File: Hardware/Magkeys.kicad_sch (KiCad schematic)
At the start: 206 parts, among them J1 Conn_01x04_Pin, SW1 SW_Push, SW10 SW_Push, SW100 SW_Push, SW101 SW_Push, SW102 RotaryEncoder, SW11 SW_Push, SW12 SW_Push, SW13 SW_Push, SW14 SW_Push, SW15 SW_Push, SW16 SW_Push, SW17 SW_Push, SW18 SW_Push, SW19 SW_Push, SW2 SW_Push, SW20 SW_Push, SW21 SW_Push, SW22 SW_Push, SW23 SW_Push, SW24 SW_Push, SW25 SW_Push, SW26 SW_Push, SW27 SW_Push, SW28 SW_Push, SW29 SW_Push, SW3 SW_Push, SW30 SW_Push, SW31 SW_Push, SW32 SW_Push, SW33 SW_Push, SW34 SW_Push, SW35 SW_Push, SW36 SW_Push, SW37 SW_Push, SW38 SW_Push, SW39 SW_Push, SW4 SW_Push, SW40 SW_Push, SW41 SW_Push, SW42 SW_Push, SW43 SW_Push, SW44 SW_Push, SW45 SW_Push, SW46 SW_Push, SW47 SW_Push, SW48 SW_Push, SW49 SW_Push, SW5 SW_Push, SW50 SW_Push, SW51 SW_Push, SW52 SW_Push, SW53 SW_Push, SW54 SW_Push, SW55 SW_Push, SW56 SW_Push, SW57 SW_Push, SW58 SW_Push, SW59 SW_Push, SW6 SW_Push, SW60 SW_Push, SW61 SW_Push, SW62 SW_Push, SW63 SW_Push, SW64 SW_Push, SW65 SW_Push, SW66 SW_Push, SW67 SW_Push, SW68 SW_Push, SW69 SW_Push, SW7 SW_Push, SW70 SW_Push, SW71 SW_Push, SW72 SW_Push, SW73 SW_Push, SW74 SW_Push, SW75 SW_Push, SW76 SW_Push, SW77 SW_Push, SW78 SW_Push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

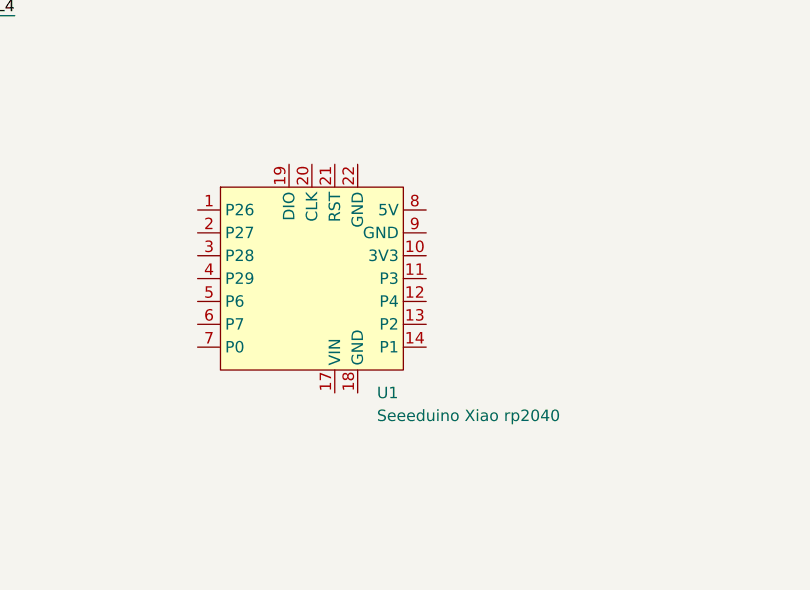
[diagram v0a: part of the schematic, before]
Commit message: Updated sch
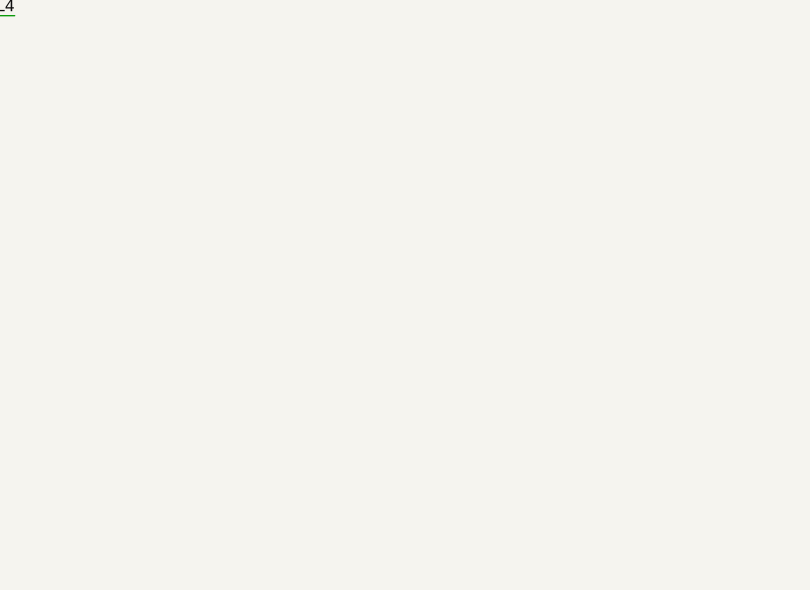
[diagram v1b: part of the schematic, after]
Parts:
- removed U1: Seeeduino Xiao rp2040, PCM_marbastlib-xp-promicroish:Xiao_rp2040_AC_Reflow, symbol PCM_marbastlib-promicroish:Seeeduino_Xiao_rp2040
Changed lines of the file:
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@@
-	)
-	(symbol
-		(lib_id "PCM_marbastlib-promicroish:Seeeduino_Xiao_rp2040")
-		(at 203.2 260.35 0)
-		(unit 1)
-		(body_style 1)
-		(exclude_from_sim no)
-		(in_bom no)
-		(on_board yes)
-		(in_pos_files yes)
-		(dnp no)
-		(fields_autoplaced yes)
-		(property "Reference" "U1"
-			(at 210.4233 273.05 0)
-			(show_name no)
-			(do_not_autoplace no)
-			(effects
-				(font
-					(size 1.27 1.27)
-				)
-				(justify left)
-			)
-		)
-		(property "Value" "Seeeduino Xiao rp2040"
-			(at 210.4233 275.59 0)
-			(show_name no)
-			(do_not_autoplace no)
-			(effects
-				(font
-					(size 1.27 1.27)
-				)
-				(justify left)
-			)
-		)
-		(property "Footprint" "PCM_marbastlib-xp-promicroish:Xiao_rp2040_AC_Reflow"
-			(at 203.2 290.83 0)
-			(hide yes)
-			(show_name no)
-			(do_not_autoplace no)
-			(effects
-				(font
-					(size 1.27 1.27)
-				)
-			)
-		)
-		(property "Datasheet" ""
-			(at 190.5 252.73 0)
-			(hide yes)
-			(show_name no)
-			(do_not_autoplace no)
-			(effects
-				(font
-					(size 1.27 1.27)
-				)
-			)
-		)
-		(property "Description" "Symbol for a Seeeduino Xiao rp2040"
-			(at 203.2 260.35 0)
-			(hide yes)
-			(show_name no)
-			(do_not_autoplace no)
-			(effects
-				(font
-					(size 1.27 1.27)
-				)
-			)
-		)
-		(pin "12"
-		)
-		(pin "14"
-		)
-		(pin "18"
-		)
-		(pin "20"
-		)
-		(pin "6"
-		)
-		(pin "5"
-		)
-		(pin "7"
-		)
-		(pin "8"
-		)
-		(pin "4"
-		)
-		(pin "9"
-		)
-		(pin "2"
-		)
-		(pin "10"
-		)
-		(pin "1"
-		)
-		(pin "3"
-		)
-		(pin "11"
-		)
-		(pin "13"
-		)
-		(pin "17"
-		)
-		(pin "19"
-		)
-		(pin "21"
-		)
-		(pin "22"
-		)
-		(instances
-			(project "Magkeys"
-				(path "/f5fc63b7-3839-4570-850a-efa69c2c2074"
-					(reference "U1")
-					(unit 1)
-				)
-			)
-		)
 	)
 	(symbol

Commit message: added a symbol
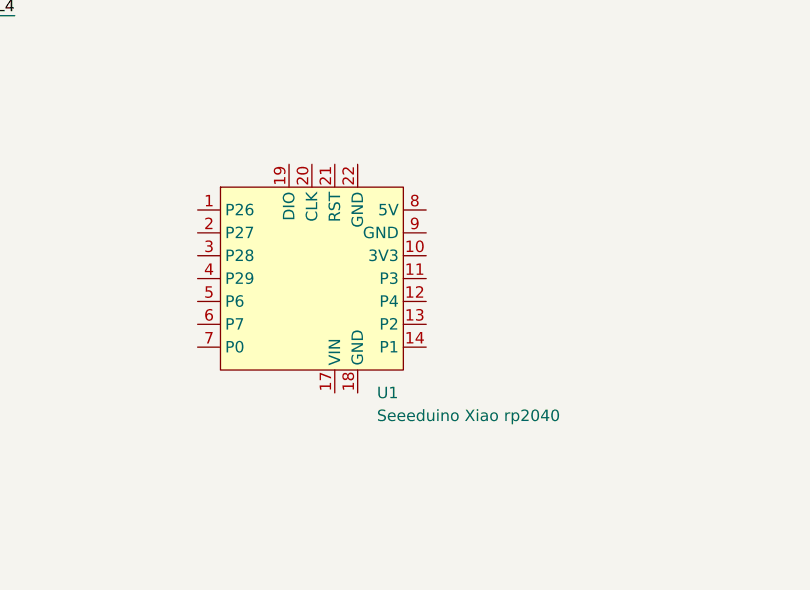
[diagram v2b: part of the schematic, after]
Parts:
- added U1: Seeeduino Xiao rp2040, PCM_marbastlib-xp-promicroish:Xiao_rp2040_AC_Reflow, symbol PCM_marbastlib-promicroish:Seeeduino_Xiao_rp2040
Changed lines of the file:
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@@
+	)
+	(symbol
+		(lib_id "PCM_marbastlib-promicroish:Seeeduino_Xiao_rp2040")
+		(at 203.2 260.35 0)
+		(unit 1)
+		(body_style 1)
+		(exclude_from_sim no)
+		(in_bom no)
+		(on_board yes)
+		(in_pos_files yes)
+		(dnp no)
+		(fields_autoplaced yes)
+		(property "Reference" "U1"
+			(at 210.4233 273.05 0)
+			(show_name no)
+			(do_not_autoplace no)
+			(effects
+				(font
+					(size 1.27 1.27)
+				)
+				(justify left)
+			)
+		)
+		(property "Value" "Seeeduino Xiao rp2040"
+			(at 210.4233 275.59 0)
+			(show_name no)
+			(do_not_autoplace no)
+			(effects
+				(font
+					(size 1.27 1.27)
+				)
+				(justify left)
+			)
+		)
+		(property "Footprint" "PCM_marbastlib-xp-promicroish:Xiao_rp2040_AC_Reflow"
+			(at 203.2 290.83 0)
+			(hide yes)
+			(show_name no)
+			(do_not_autoplace no)
+			(effects
+				(font
+					(size 1.27 1.27)
+				)
+			)
+		)
+		(property "Datasheet" ""
+			(at 190.5 252.73 0)
+			(hide yes)
+			(show_name no)
+			(do_not_autoplace no)
+			(effects
+				(font
+					(size 1.27 1.27)
+				)
+			)
+		)
+		(property "Description" "Symbol for a Seeeduino Xiao rp2040"
+			(at 203.2 260.35 0)
+			(hide yes)
+			(show_name no)
+			(do_not_autoplace no)
+			(effects
+				(font
+					(size 1.27 1.27)
+				)
+			)
+		)
+		(pin "12"
+		)
+		(pin "14"
+		)
+		(pin "18"
+		)
+		(pin "20"
+		)
+		(pin "6"
+		)
+		(pin "5"
+		)
+		(pin "7"
+		)
+		(pin "8"
+		)
+		(pin "4"
+		)
+		(pin "9"
+		)
+		(pin "2"
+		)
+		(pin "10"
+		)
+		(pin "1"
+		)
+		(pin "3"
+		)
+		(pin "11"
+		)
+		(pin "13"
+		)
+		(pin "17"
+		)
+		(pin "19"
+		)
+		(pin "21"
+		)
+		(pin "22"
+		)
+		(instances
+			(project "Magkeys"
+				(path "/f5fc63b7-3839-4570-850a-efa69c2c2074"
+					(reference "U1")
+					(unit 1)
+				)
+			)
+		)
 	)
 	(symbol
